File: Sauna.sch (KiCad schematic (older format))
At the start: 8 parts, among them J1 Barrel_Jack_MountingPin, J2 Screw_Terminal_01x02, J3 Screw_Terminal_01x03, K1 FINDER-40.11, Q1 2N2219, U1 NodeMCU_1.0_(ESP-12E)

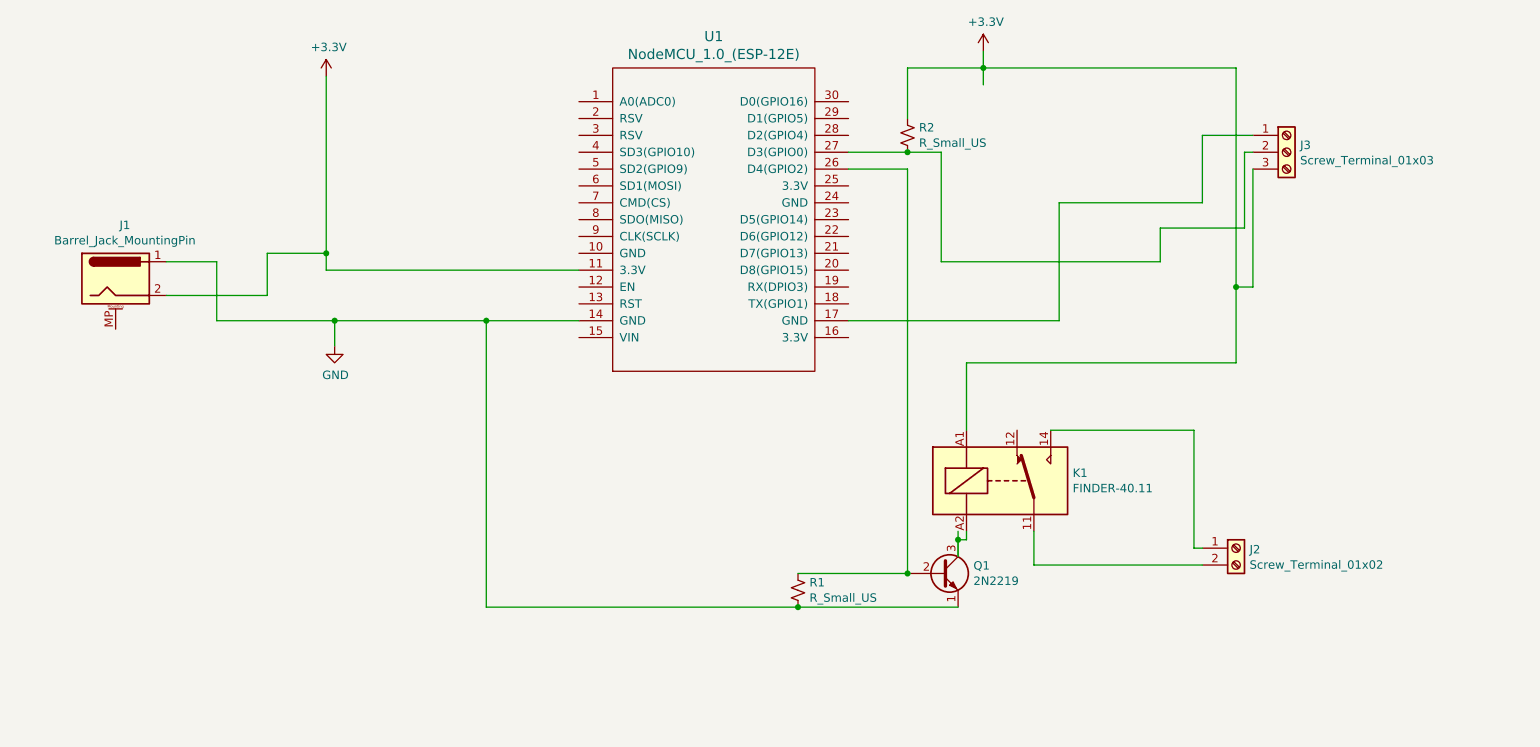
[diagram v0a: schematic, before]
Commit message: ver 0 .1
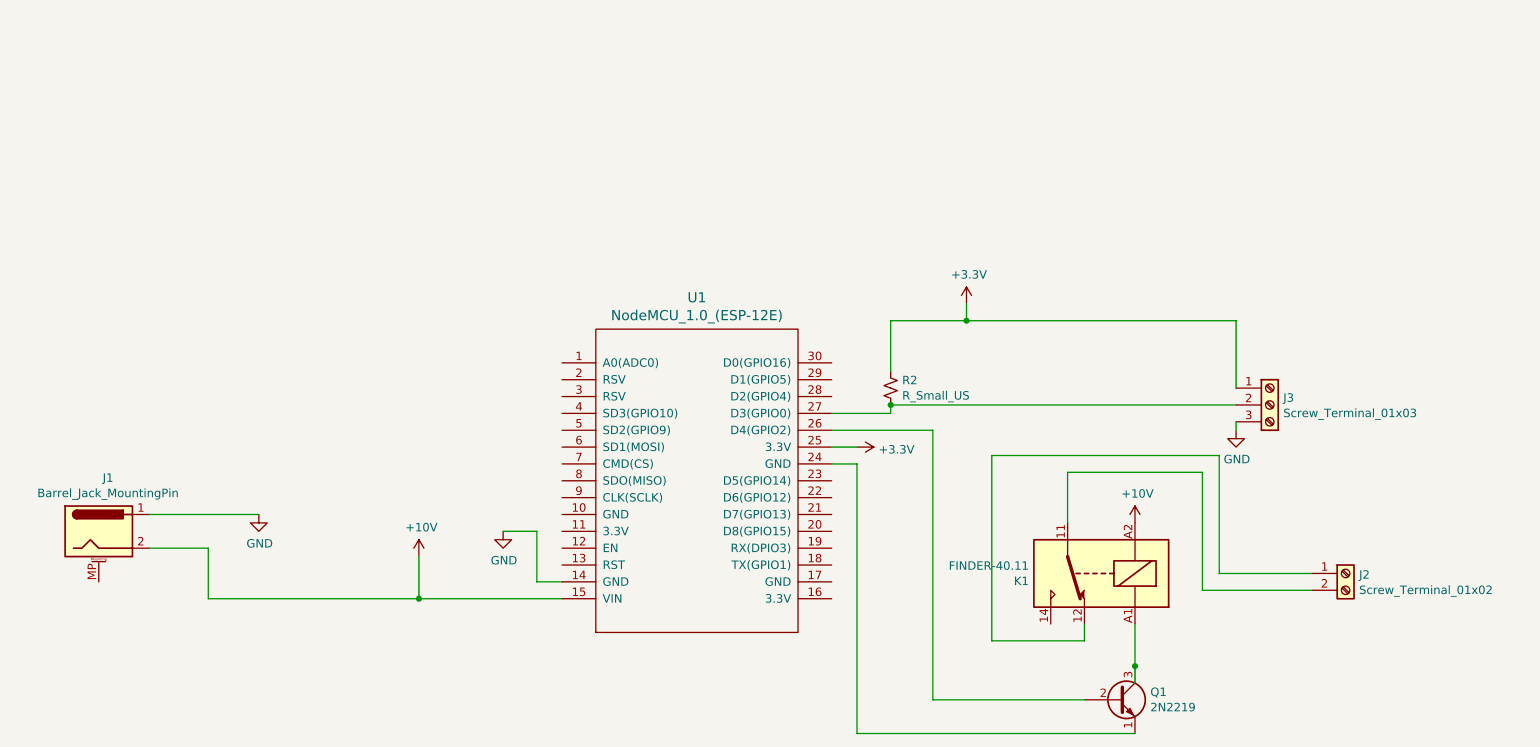
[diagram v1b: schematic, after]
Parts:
- removed R1: R_Small_US, Resistor_SMD:R_0603_1608Metric_Pad1.05x0.95mm_HandSolder, symbol Device:R_Small_US
- J3: footprint TerminalBlock_4Ucon:TerminalBlock_4Ucon_1x02_P3.50mm_Vertical -> TerminalBlock_4Ucon:TerminalBlock_4Ucon_1x03_P3.50mm_Vertical
- U1: footprint (none) -> ESP8266:NodeMCU1.0(12-E)
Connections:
- net labels added: +10V
- wire segments 51 -> 37
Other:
- moved on the sheet: J1, J2, J3, K1, Q1, R2, U1
